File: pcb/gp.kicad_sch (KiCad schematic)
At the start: 31 parts, among them J1 USB-C, SW1 TS-1088R-02526, SW2 TS-1088R-02526, U1 XC6206P332MR, U2 STM32F103CBT6, U3 W25Q128JVSIQ, Y1 16Mhz

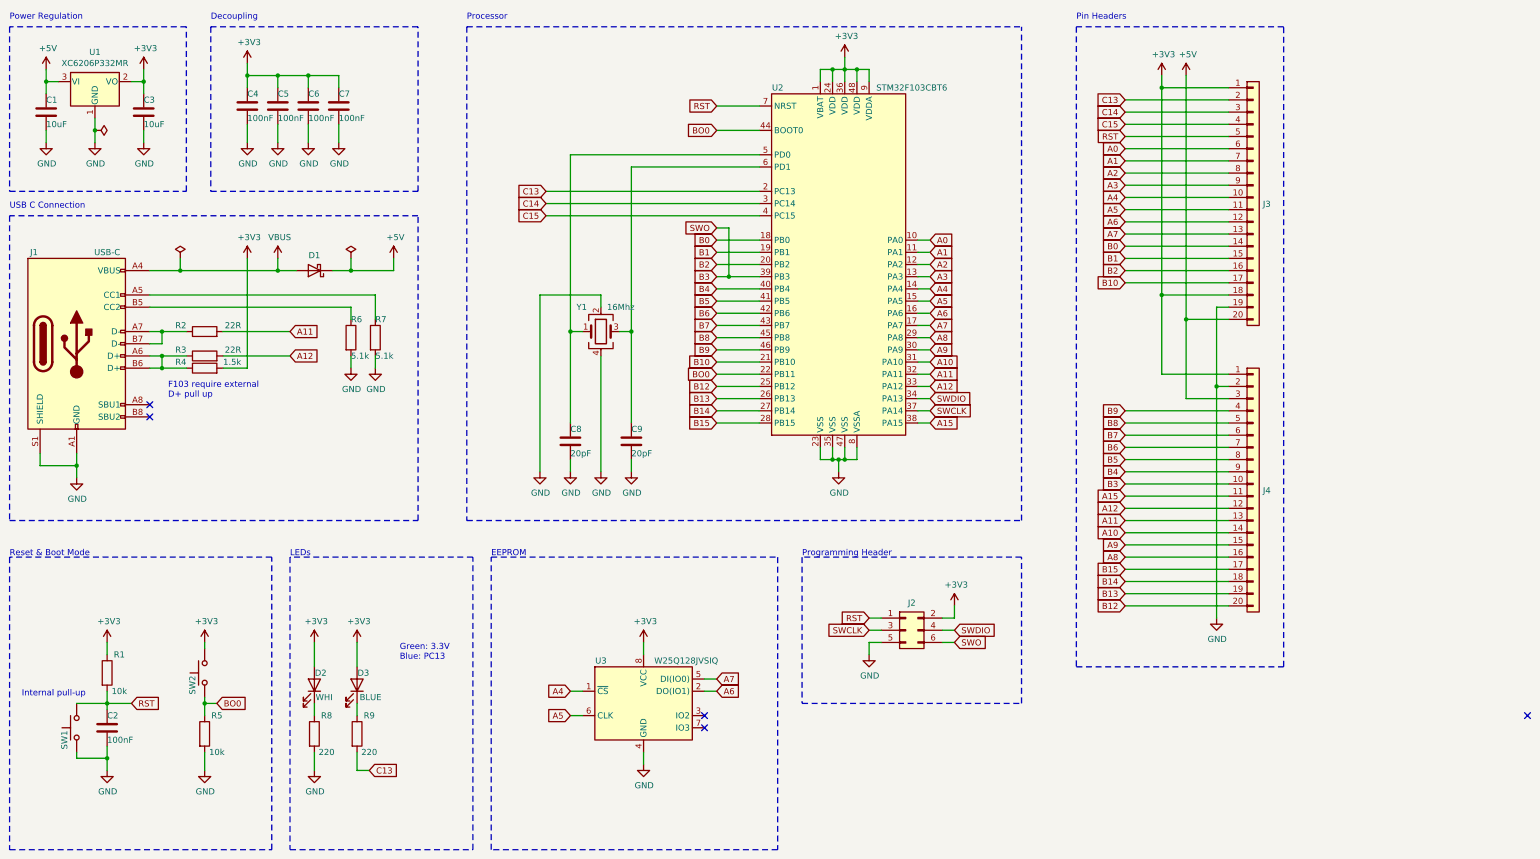
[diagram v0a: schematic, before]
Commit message: Tweaks
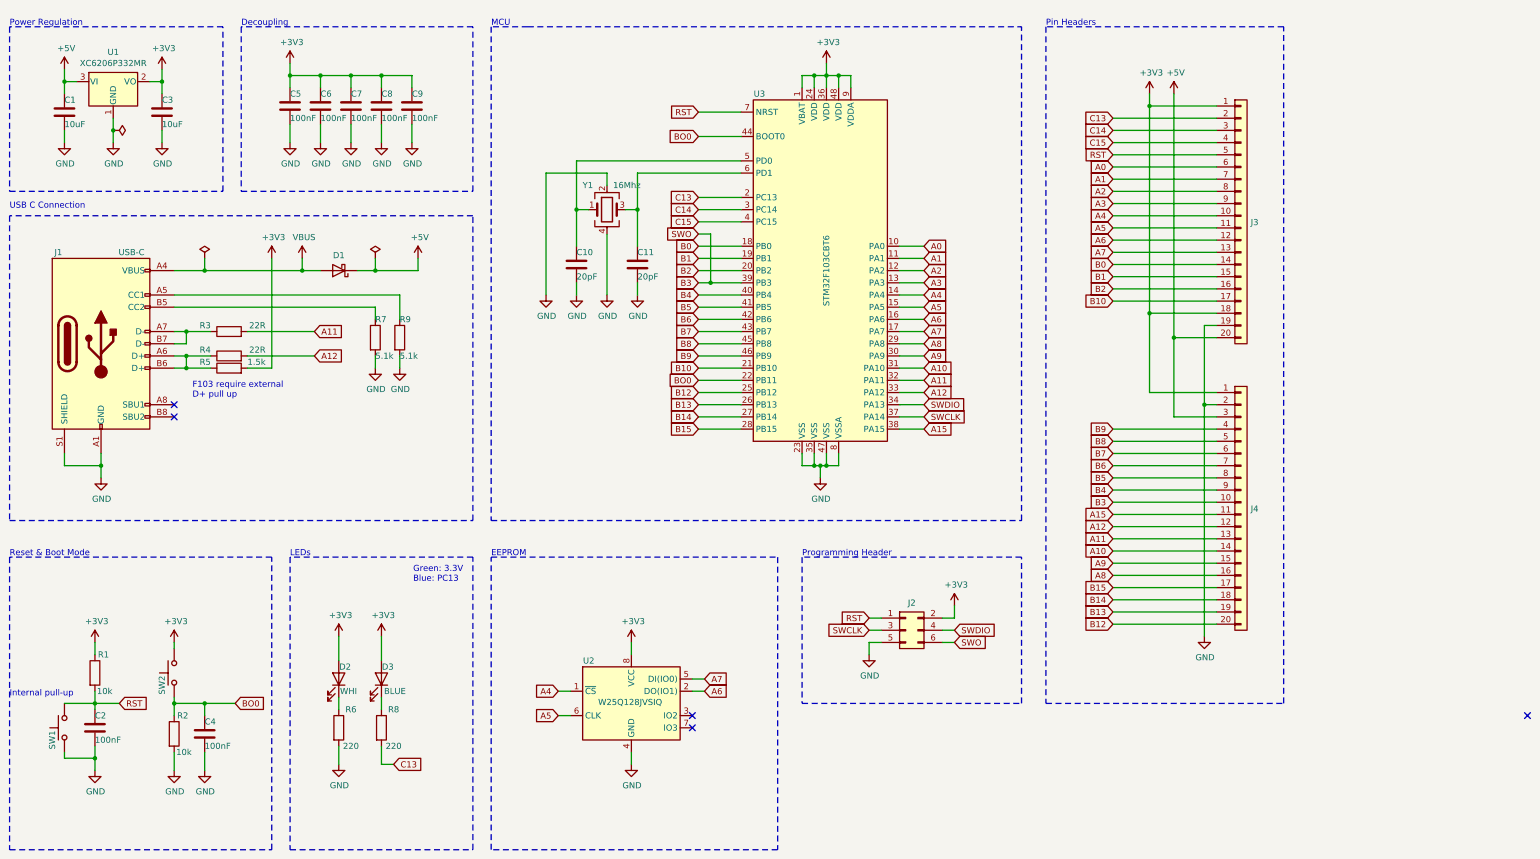
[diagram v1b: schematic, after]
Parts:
- added C4, C9: 100nF, Capacitor_SMD:C_0402_1005Metric, symbol Device:C
- renumbered C8 to C10, C9 to C11, C4 to C5, C5 to C6, C6 to C7, C7 to C8, R5 to R2, R2 to R3, R3 to R4, R4 to R5, R8 to R6, R6 to R7, R9 to R8, R7 to R9, U3 to U2, U2 to U3
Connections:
- net +3V3: now also C9.1
- net BO0: now also C4.1
- net GND: now also C4.2, C9.2
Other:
- note added: "MCU"
- note removed: "Processor"
- moved on the sheet: C1, C10, C11, C2, C3, C5, C6, C7, C8, D1, D2, D3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
